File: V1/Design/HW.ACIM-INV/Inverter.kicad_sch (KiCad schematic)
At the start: 53 parts, among them J3 MOTOR, M1 560V/1.75kA, M2 560V/1.75kA, M3 560V/1.75kA, Q4 20V/1A, Q5 20V/1A, Q6 20V/1A, U1 IPM 600V/15A

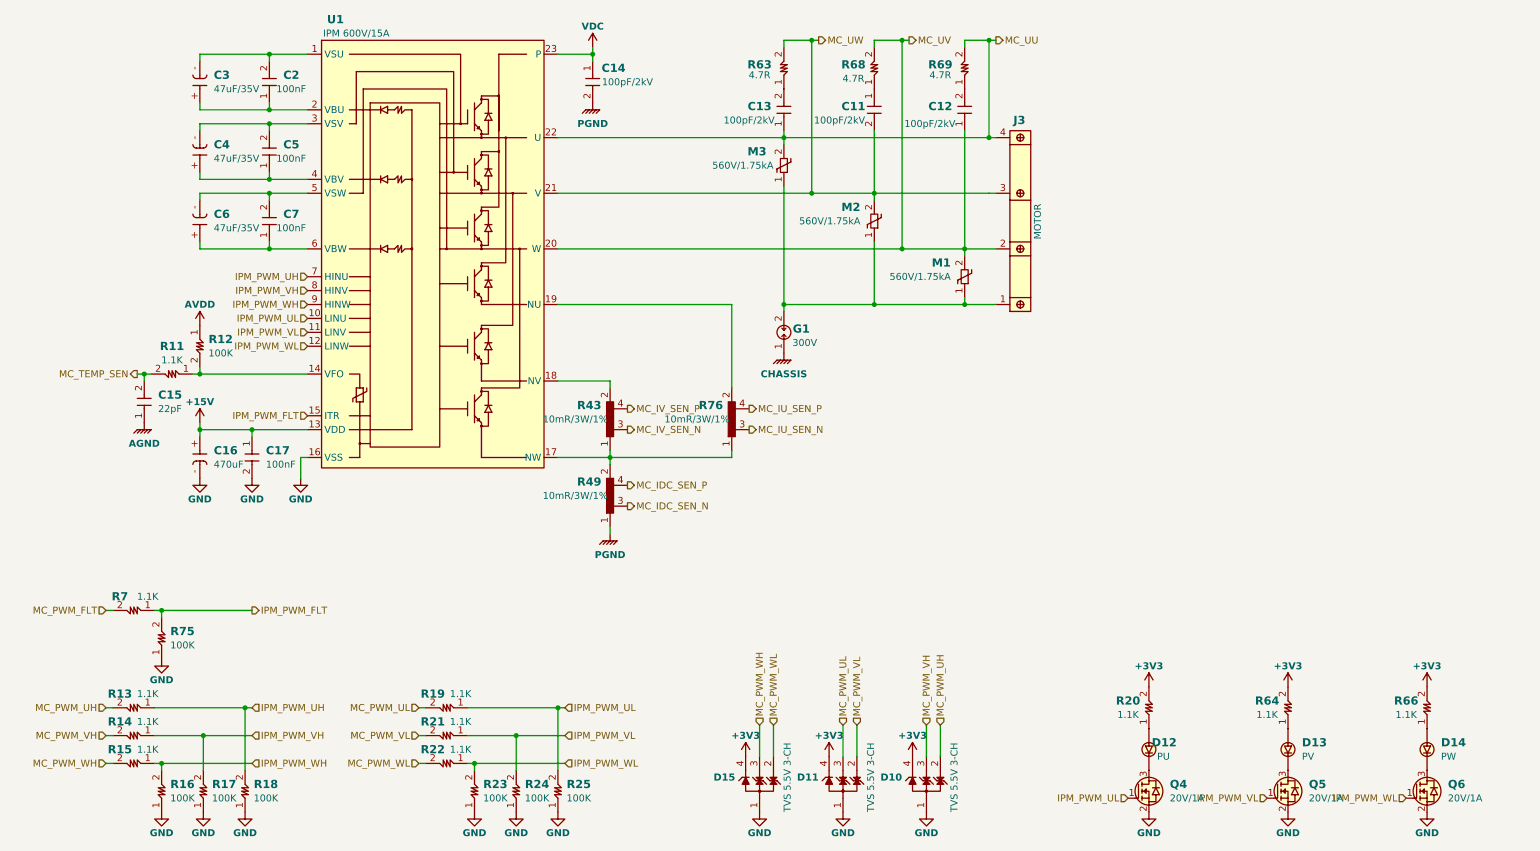
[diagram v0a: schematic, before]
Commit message: V1 schematic update 6
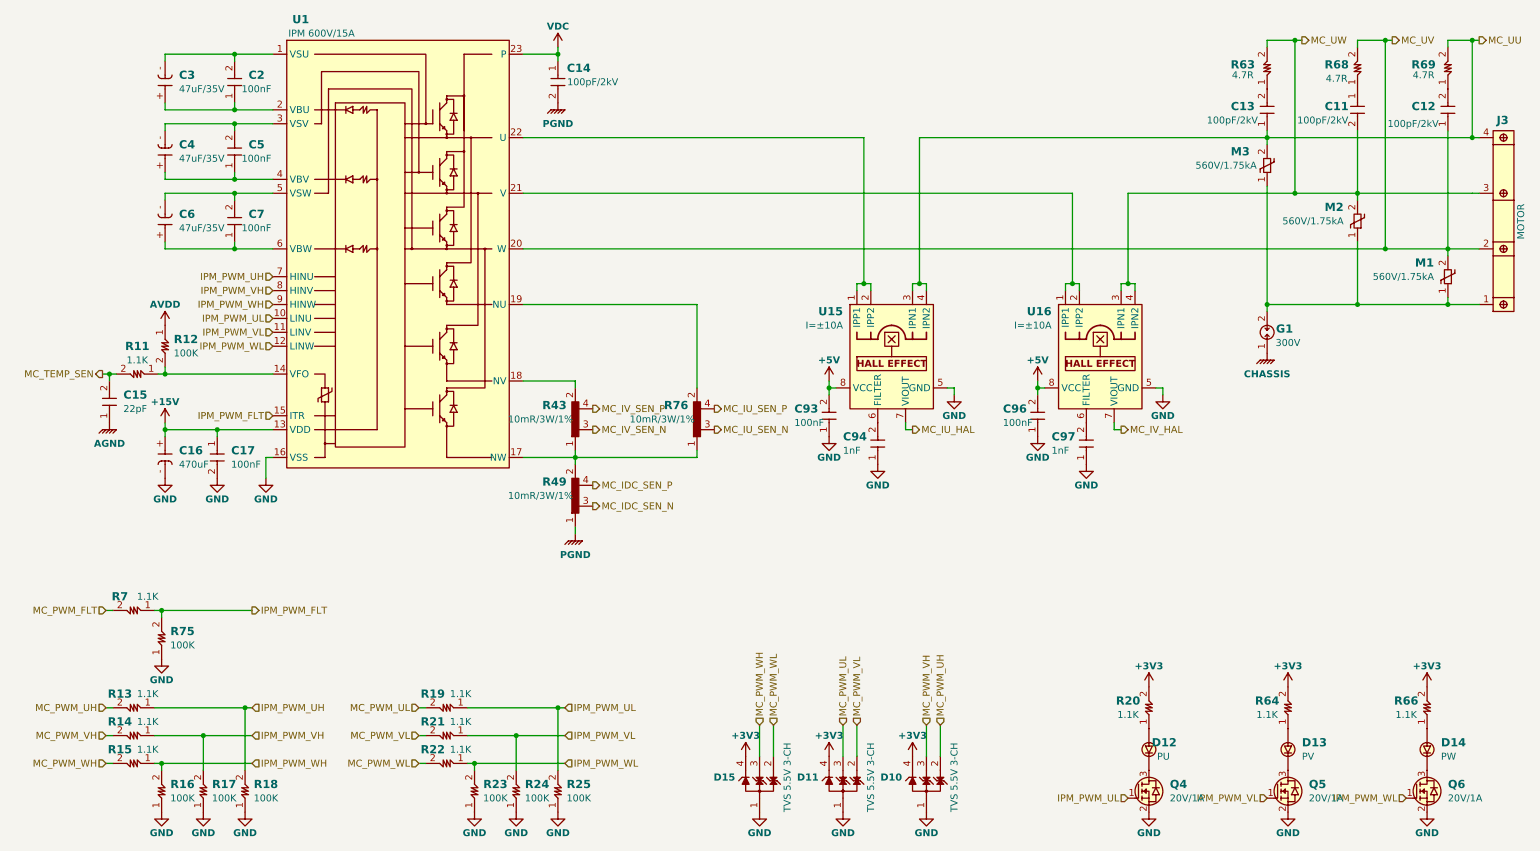
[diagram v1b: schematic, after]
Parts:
- added C93, C96: 100nF, SAMPI:CAP0603, symbol SAMPI:CERCAP
- added C94, C97: 1nF, SAMPI:CAP0603, symbol SAMPI:CERCAP
- added U15, U16: I=±10A, SAMPI:SOIC8_ALL, symbol SAMPI:ACS724
- C11, C12, C13, C14: Checked OK -> (none); Unit Price 0.19 -> (none)
- C15: Checked OK -> (none); Unit Price 0.012 -> (none)
- C16: Checked OK -> (none); Unit Price 0.85 -> (none)
- C17, C2, C5, C7: Checked OK -> (none); Unit Price 0.0146 -> (none)
- C3, C4, C6: Checked OK -> (none); Unit Price 0.45 -> (none)
- D10, D11, D13, D15: Checked OK -> (none)
- D12, D14: Checked OK -> (none); Unit Price 0.1 -> (none)
- G1: Checked OK -> (none); Unit Price 0.53 -> (none)
- J3: Checked OK -> (none); Unit Price 0.84 -> (none)
- M1, M2, M3: Checked OK -> (none); Unit Price 0.255 -> (none)
- Q4, Q5, Q6: Checked OK -> (none); Unit Price 0.148 -> (none)
- R11, R13, R14, R15, R19, R20, R21, R22, R64, R66, R7: Checked OK -> (none); Unit Price 0.021 -> (none)
- R12, R16, R17, R18, R23, R24, R25, R75: Checked OK -> (none); Unit Price 0.019 -> (none)
- R43, R49, R76: Checked OK -> (none); Unit Price 0.6 -> (none)
- R63, R68, R69: Checked OK -> (none); Unit Price 0.035 -> (none)
- U1: Checked OK -> (none); Unit Price 11.37 -> (none)
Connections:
- net GND: now also C93.1, C94.1, C96.1, C97.1, U15.5 (GND), U16.5 (GND)
- net MC_UU: now also U15.3 (IPN1), U15.4 (IPN2); no longer U1.22 (U)
- net MC_UW: now also U16.3 (IPN1), U16.4 (IPN2); no longer U1.21 (V)
- new net: C97.2, U16.6 (FILTER)
- new net: C94.2, U15.6 (FILTER)
- new net: U1.21 (V), U16.1 (IPP1), U16.2 (IPP2)
- new net: U1.22 (U), U15.1 (IPP1), U15.2 (IPP2)
- new net +5V: C93.2, C96.2, U15.8 (VCC), U16.8 (VCC)
- new net MC_IU_HAL: U15.7 (VIOUT)
- new net MC_IV_HAL: U16.7 (VIOUT)
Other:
- moved on the sheet: C11, C12, C13, C14, C15, C16, C17, C2, C3, C4, C5, C6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
